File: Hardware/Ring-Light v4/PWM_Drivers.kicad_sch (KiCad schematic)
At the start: 38 parts, among them U33 PCA9685BS,118, U34 PCA9685BS,118

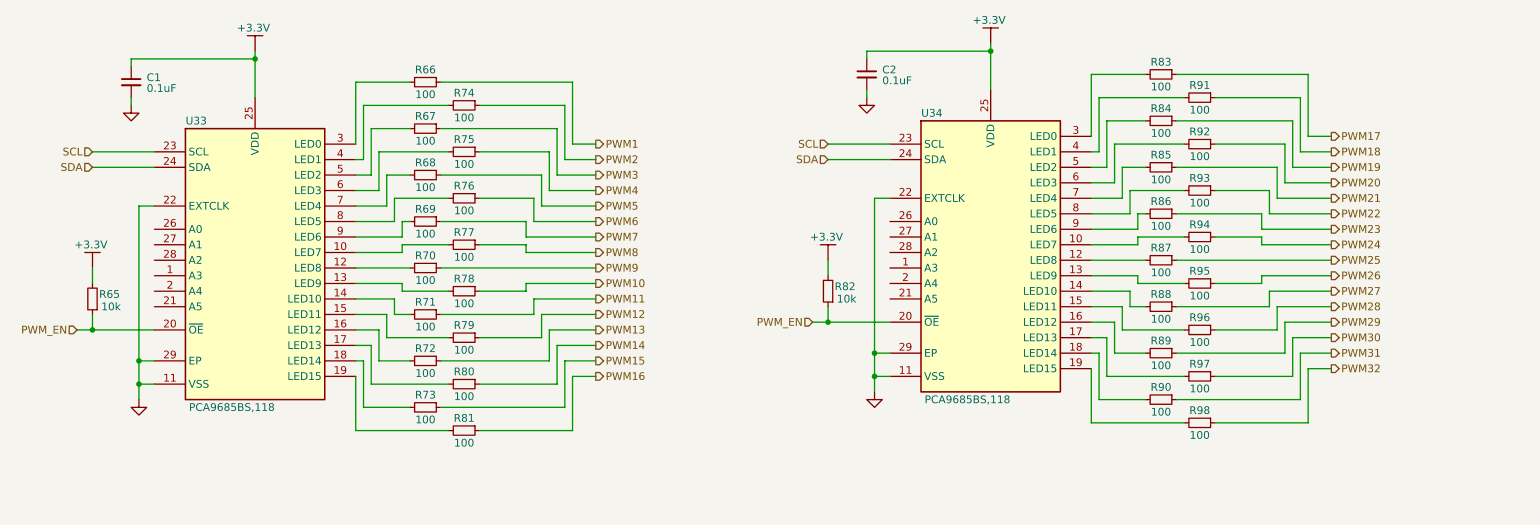
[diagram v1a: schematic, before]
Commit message: d
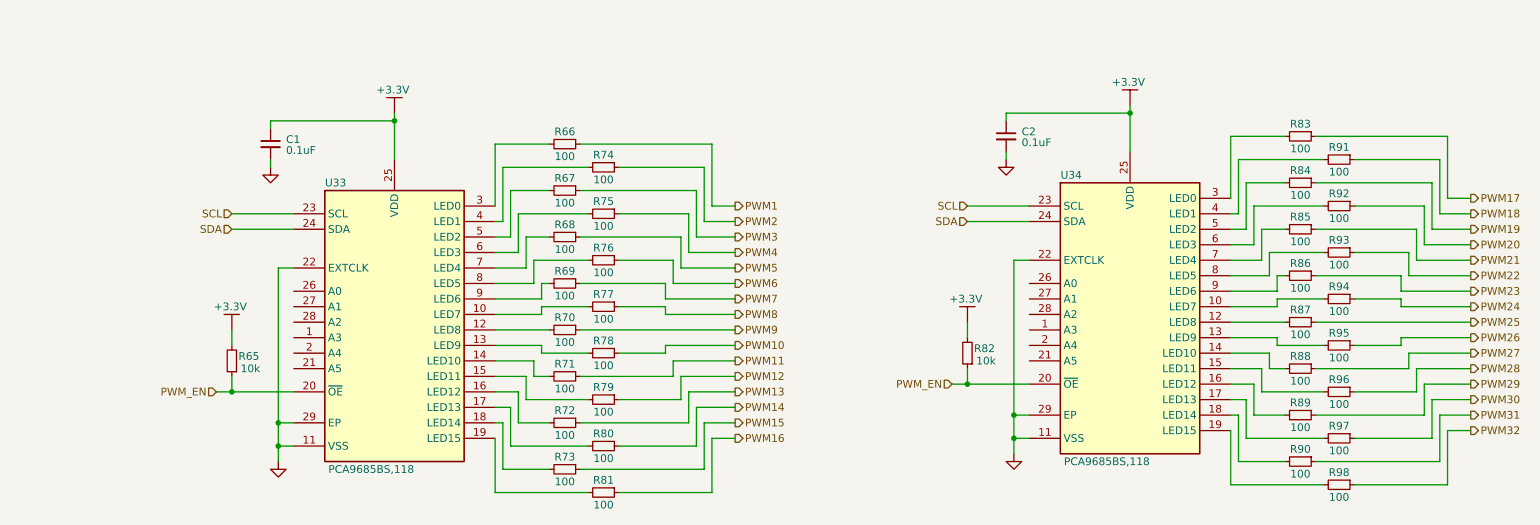
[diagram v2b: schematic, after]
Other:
- moved on the sheet: C1, C2, R65, R66, R67, R68, R69, R70, R71, R72, R73, R74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
